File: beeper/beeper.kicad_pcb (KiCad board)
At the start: 2 copper layers, 26.8 x 16.5 mm, 28 parts, among them J1 Conn_01x03, J2 TEST_1P, J3 TEST_1P, J4 TEST_1P, J5 TEST_1P, Q2 Q_NMOS_DGS, SW1 SW_Push, U1 ATTINY13A-SSU, U2 MCP73831-2-OT

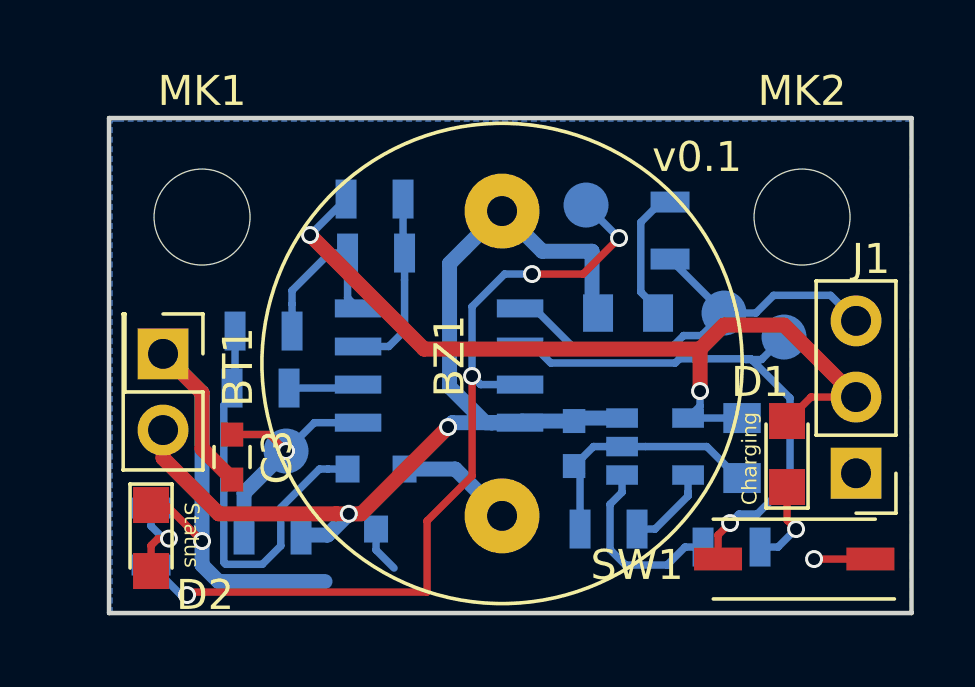
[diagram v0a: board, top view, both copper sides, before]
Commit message: Version 2.
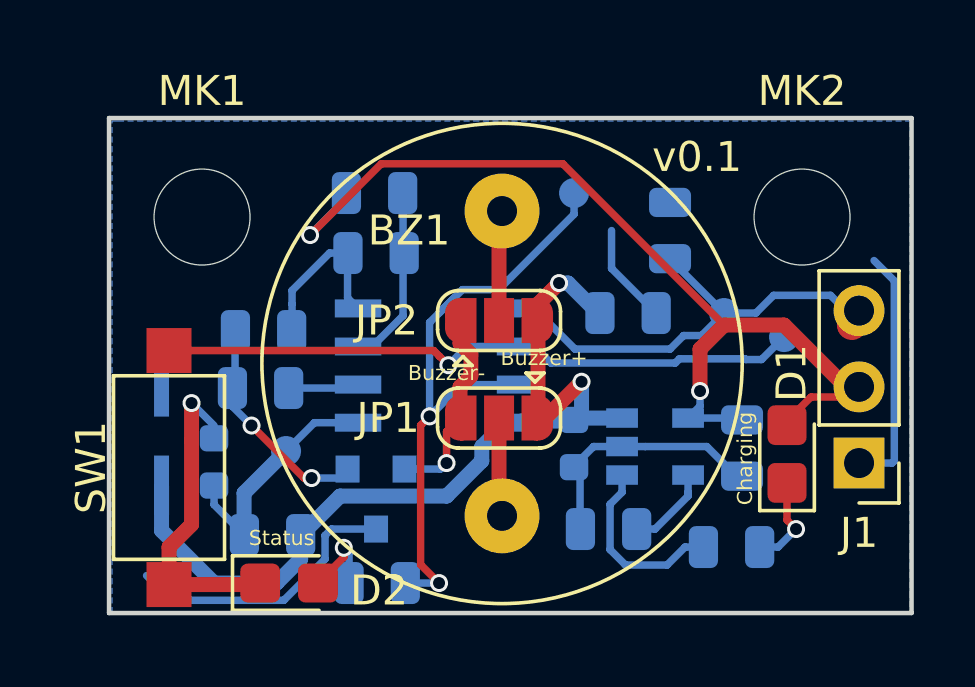
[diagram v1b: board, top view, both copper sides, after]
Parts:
- added JP1: Jumper_NC_Dual, Jumper:SolderJumper-3_P1.3mm_Open_RoundedPad1.0x1.5mm, F.Cu at (149.5, 104.5)
- added JP2: Jumper_NC_Dual, Jumper:SolderJumper-3_P1.3mm_Open_RoundedPad1.0x1.5mm, F.Cu at (149.5, 101.2)
- BT1: footprint Pin_Headers:Pin_Header_Straight_2x01_Pitch2.54mm -> Connector_PinHeader_1.00mm:PinHeader_2x01_P1.00mm_Vertical_SMD; moved to B.Cu
- C1, C4: footprint Capacitors_SMD:C_0805 -> Capacitor_SMD:C_0805_2012Metric
- C2: footprint Capacitors_SMD:C_0603 -> Capacitor_SMD:C_0603_1608Metric
- C3: footprint Capacitors_SMD:C_0603 -> Capacitor_SMD:C_0603_1608Metric; moved to B.Cu
- D1, D2: footprint LEDs:LED_0805 -> LED_SMD:LED_0805_2012Metric_Castellated
- J1: footprint Pin_Headers:Pin_Header_Straight_1x03_Pitch2.54mm -> Connector_PinHeader_2.54mm:PinHeader_1x03_P2.54mm_Vertical
- J2, J3, J4, J5: footprint Measurement_Points:Measurement_Point_Round-SMD-Pad_Small -> TestPoint:TestPoint_Pad_D1.0mm
- MK1, MK2: footprint Mounting_Holes:MountingHole_3.2mm_M3 -> MountingHole:MountingHole_3.2mm_M3
- Q2: footprint TO_SOT_Packages_SMD:SOT-23 -> Package_TO_SOT_SMD:SOT-23
- R1, R2, R3, R4, R5, R6, R7, R8, R9: footprint Resistors_SMD:R_0805 -> Resistor_SMD:R_0805_2012Metric
- SW1: footprint Buttons_Switches_SMD:SW_DIP_x1_W5.08mm_Slide_Copal_CHS-A -> Button_Switch_SMD:SW_SPST_CK_RS282G05A3
- U1: footprint Housings_SOIC:SOIC-8_3.9x4.9mm_Pitch1.27mm -> Package_SO:SOIC-8_3.9x4.9mm_P1.27mm
- U2: footprint TO_SOT_Packages_SMD:SOT-23-5 -> Package_TO_SOT_SMD:SOT-23-5
- moved SW1 21.1 mm to (138.5, 106.2), turned to 90 degrees
- moved R9 7.70 mm to (145.4, 110.0), turned to 180 degrees
- moved D2 4.84 mm to (142.5, 110.0), turned to 0 degrees
- moved BT1 2.74 mm to (138.2, 105.1)
- moved C3 0.62 mm to (140.0, 106.0), turned to 270 degrees
- moved J5 0.57 mm to (152.0, 97.0)
- moved J1 0.35 mm to (161.5, 106.0)
- moved R2 0.20 mm to (145.3, 97.0)
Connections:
- BZ1 pad 2: VCC -> Net-(BZ1-Pad2)
- Q2 pad 2: Net-(BZ1-Pad1) -> /BUZZER_GND
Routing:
- net /STATUS_OUT: track 28.9 -> 21.4 mm, vias 4 -> 2
- net /BUZZER_GND: track 0.00 -> 6.77 mm, vias 0 -> 1
- net Net-(Q2-Pad1): track 13.6 -> 7.36 mm, vias 0 -> 2
- net VCC: track 36.2 -> 31.0 mm
- net GND: track 43.4 -> 47.7 mm, vias 2 -> 1
- net Net-(BZ1-Pad2): track 0.00 -> 3.69 mm
- net Net-(J4-Pad1): track 18.2 -> 21.6 mm
- net +5V: track 30.2 -> 32.6 mm
- net /sense: track 6.65 -> 5.81 mm
- net Net-(BZ1-Pad1): track 4.57 -> 3.92 mm
- net Net-(C3-Pad2): track 8.20 -> 7.99 mm, vias 1 -> 0
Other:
- rule trace_min: 0.1524 -> 0.2
- board text added: "Buzzer+"
- board text added: "Buzzer-"
- board text removed: "Beep-"
- board text removed: "VCC"

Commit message: PCB v0.2
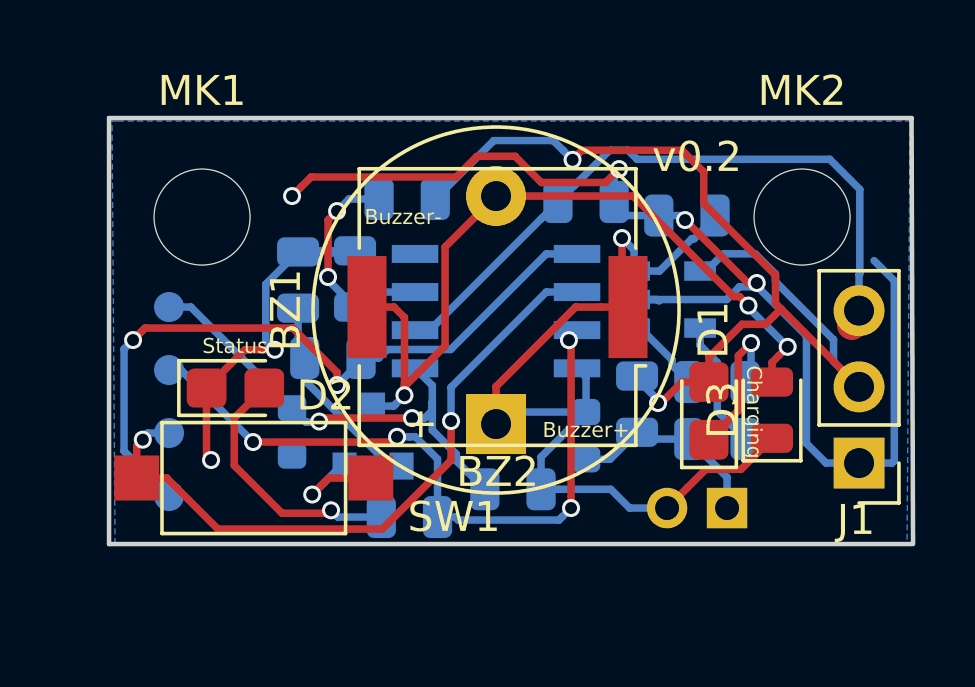
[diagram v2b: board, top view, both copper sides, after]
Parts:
- removed JP1, JP2: Jumper_NC_Dual, Jumper:SolderJumper-3_P1.3mm_Open_RoundedPad1.0x1.5mm
- added BZ2: Buzzer, Buzzer_Beeper:Buzzer_Murata_PKMCS0909E4000-R1, F.Cu at (149.4, 100.8)
- added D3: D, Diode_SMD:D_0805_2012Metric, F.Cu at (158.6, 104.2)
- BT1: footprint Connector_PinHeader_1.00mm:PinHeader_2x01_P1.00mm_Vertical_SMD -> Connector_PinHeader_2.00mm:PinHeader_2x01_P2.00mm_Vertical
- BZ1: footprint Buzzers_Beepers:BUZZER -> Buzzer_Beeper:Buzzer_12x9.5RM7.6
- J2: value TEST_1P -> SCK
- J3: value TEST_1P -> MISO
- J4: value TEST_1P -> RST
- J5: value TEST_1P -> MOSI
- Q2: value Q_NMOS_DGS -> irlml2502
- R4: value 100k -> 10k
- moved J4 20.5 mm to (138.5, 100.8)
- moved BT1 19.0 mm to (157.1, 107.5), turned to 180 degrees
- moved J2 18.6 mm to (138.5, 102.9)
- moved J5 16.9 mm to (138.5, 107.1)
- moved R7 8.16 mm to (150.0, 106.9)
- moved D2 6.74 mm to (140.7, 103.5)
- moved R8 5.52 mm to (156.8, 103.3)
- moved U2 4.92 mm to (155.1, 100.5)
- moved R1 4.70 mm to (156.8, 105.2)
- moved J3 3.95 mm to (138.5, 105.0)
- moved C1 3.80 mm to (155.8, 97.8), turned to 180 degrees
- moved C4 3.79 mm to (154.1, 104.0)
- moved D1 2.97 mm to (156.5, 104.3)
- moved R6 2.96 mm to (152.4, 97.3), turned to 0 degrees
- moved SW1 2.85 mm to (141.3, 106.5), turned to 180 degrees
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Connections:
- BZ1 pad 1: Net-(BZ1-Pad1) -> VCC
- BZ1 pad 2: Net-(BZ1-Pad2) -> /BUZZER_GND
- J2 pad 1: /Beeper_in -> /STATUS_OUT
- J3 pad 1: Net-(C3-Pad2) -> Net-(J3-Pad1)
- J4 pad 1: Net-(J4-Pad1) -> Net-(C3-Pad2)
- J5 pad 1: /STATUS_OUT -> /BUZZER_OUT
- Q2 pad 2: /BUZZER_GND -> GND
- Q2 pad 3: GND -> /BUZZER_GND
- SW1 pad 2: Net-(J4-Pad1) -> Net-(J3-Pad1)
- U1 pad 2: /BUZZER_OUT -> /Beeper_in
- U1 pad 5: /Beeper_in -> /BUZZER_OUT
- U1 pad 6: Net-(J4-Pad1) -> Net-(J3-Pad1)
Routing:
- net Net-(J3-Pad1): track 0.00 -> 22.4 mm, vias 0 -> 2
- net /BUZZER_OUT: track 2.35 -> 24.5 mm, vias 0 -> 2
- net Net-(J4-Pad1): track 21.6 -> 0.00 mm, vias 1 -> 0
- net /BUZZER_GND: track 6.77 -> 26.7 mm, vias 1 -> 3
- net GND: track 47.7 -> 62.2 mm, vias 1 -> 7
- net Net-(C3-Pad2): track 7.99 -> 16.0 mm, vias 0 -> 2
- net /Beeper_in: track 16.0 -> 22.1 mm
- net Net-(D2-Pad2): track 2.78 -> 8.69 mm
- net Net-(BZ1-Pad1): track 3.92 -> 0.00 mm
- net Net-(BZ1-Pad2): track 3.69 -> 0.00 mm
- net Net-(R8-Pad2): track 6.21 -> 2.68 mm
- net +5V: track 32.6 -> 35.7 mm
- net Net-(D1-Pad1): track 2.97 -> 5.29 mm
- net /STATUS_OUT: track 21.4 -> 23.2 mm, vias 2 -> 4
- net /sense: track 5.81 -> 7.47 mm, vias 0 -> 2
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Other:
- board size 26.8 x 16.5 mm -> 26.8 x 14.2 mm
- board text added: "v0.2"
- board text removed: "v0.1"

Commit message: PCB v0.2 final
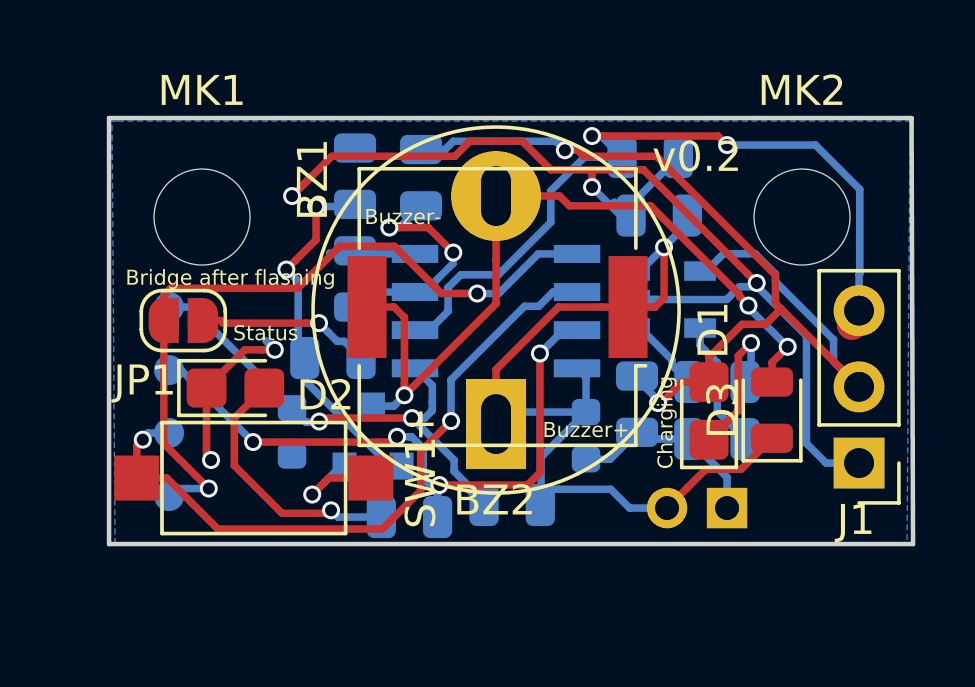
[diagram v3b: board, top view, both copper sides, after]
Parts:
- added JP1: enable buzzer, Jumper:SolderJumper-2_P1.3mm_Open_RoundedPad1.0x1.5mm, F.Cu at (139.0, 101.2)
- BZ1: footprint Buzzer_Beeper:Buzzer_12x9.5RM7.6 -> buzzer:Buzzer_12x9.5RM7.6_oval3
- moved R4 3.95 mm to (144.7, 96.4)
- moved R6 2.61 mm to (154.5, 95.8)
- moved C1 0.92 mm to (154.8, 97.8)
- moved R2 0.85 mm to (146.9, 96.5), turned to 270 degrees
- moved R7 0.53 mm to (149.9, 107.4)
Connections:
- J5 pad 1: /BUZZER_OUT -> Net-(J5-Pad1)
- U1 pad 5: /BUZZER_OUT -> Net-(J5-Pad1)
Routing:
- net Net-(J5-Pad1): track 0.00 -> 24.1 mm, vias 0 -> 2
- net /BUZZER_OUT: track 24.5 -> 6.09 mm, vias 2 -> 1
- net GND: track 62.2 -> 56.0 mm, vias 7 -> 6
- net Net-(Q2-Pad1): track 7.34 -> 12.6 mm, vias 0 -> 2
- net /Beeper_in: track 22.1 -> 26.3 mm, vias 0 -> 2
- net +5V: track 35.7 -> 34.6 mm
- net /STATUS_OUT: track 23.2 -> 22.5 mm
- net /sense: track 7.47 -> 8.07 mm
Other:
- board text added: "Bridge after flashing"

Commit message: Final v0.2 (ordered)
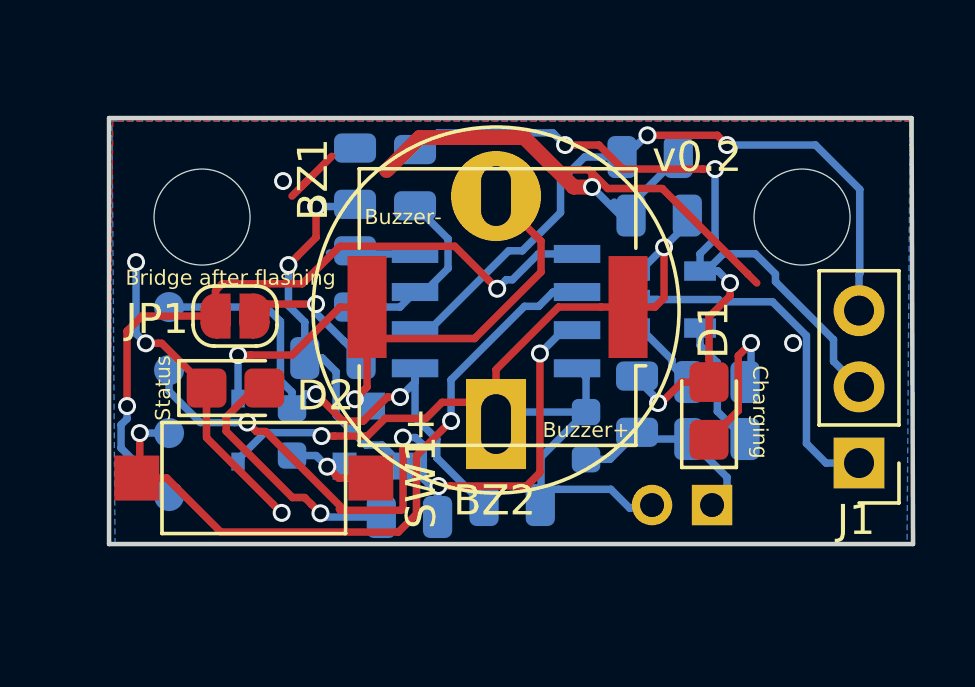
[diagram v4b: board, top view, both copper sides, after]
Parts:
- D3: value D -> 1N4148; footprint Diode_SMD:D_0805_2012Metric -> Diode_SMD:D_SOD-323; moved to B.Cu
- moved D3 17.8 mm to (140.8, 104.9)
- moved JP1 1.73 mm to (140.7, 101.1)
- moved BT1 0.51 mm to (156.6, 107.4)
- moved R2 0.20 mm to (146.7, 96.5)
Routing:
- net /BUZZER_GND: track 26.8 -> 21.0 mm, vias 3 -> 2
- net VCC: track 33.0 -> 38.4 mm, vias 1 -> 2
- net GND: track 56.0 -> 60.6 mm, vias 6 -> 7
- net /STATUS_OUT: track 22.5 -> 26.4 mm
- net +5V: track 34.6 -> 31.0 mm, vias 2 -> 4
- net Net-(C3-Pad2): track 16.1 -> 18.9 mm
- net /Beeper_in: track 26.3 -> 23.7 mm
- net /sense: track 8.07 -> 6.18 mm, vias 2 -> 0
- net Net-(J3-Pad1): track 22.6 -> 23.2 mm
- added copper zone on F.Cu, net GND
